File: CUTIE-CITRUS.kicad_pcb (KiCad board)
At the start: 2 copper layers, 31 parts, among them J1 F32Q-1A7H1-11022, J2 F32Q-1A7H1-11022, J3 Bus_M.2_Socket_M, U1 ASEK-32.768KHZ-L-R-T, U2 AP3441SHE-7B, U3 ICM-42688-P, U4 NEO-M8M

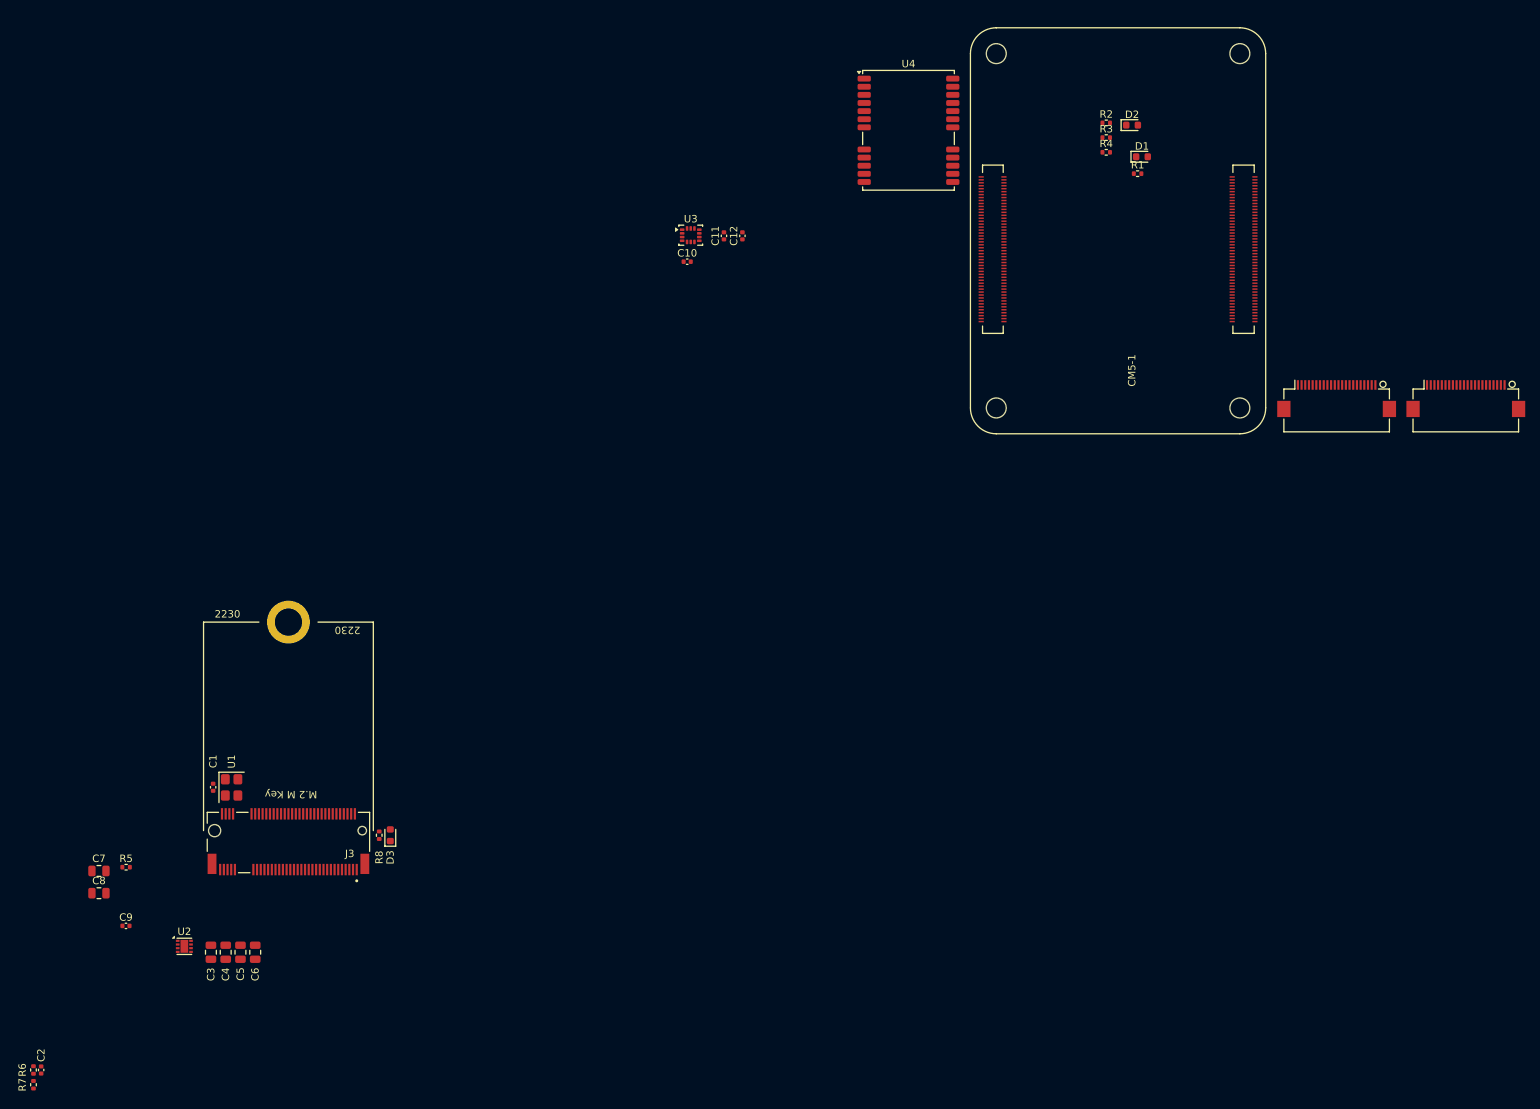
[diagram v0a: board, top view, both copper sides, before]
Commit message: neo m8m impl.
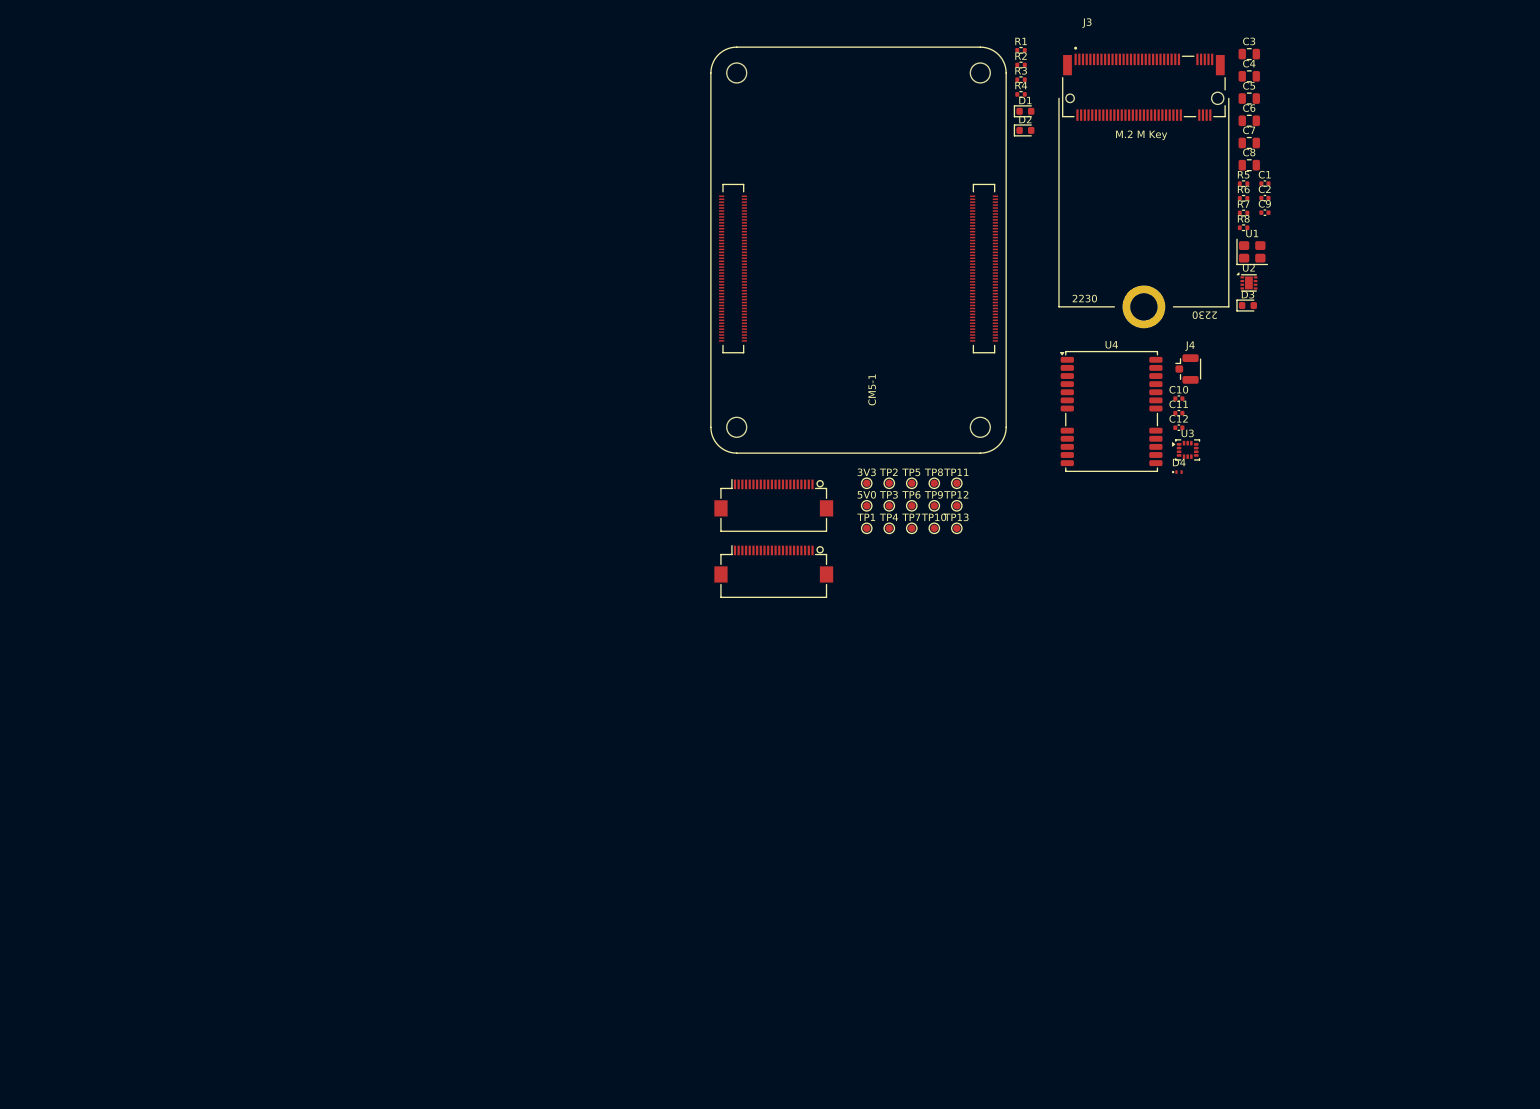
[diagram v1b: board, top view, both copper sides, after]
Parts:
- added 3V3: TestPoint, TestPoint:TestPoint_Pad_D1.0mm, F.Cu at (136.3, 110.5)
- added 5V0: TestPoint, TestPoint:TestPoint_Pad_D1.0mm, F.Cu at (136.3, 113.6)
- added D4: TPD1E05U06DPY, Package_SON:Texas_DPY0002A_0.6x1mm_P0.65mm, F.Cu at (178.7, 109.0)
- added J4: Hirose U.FL, Connector_Coaxial:U.FL_Hirose_U.FL-R-SMT-1_Vertical, F.Cu at (179.7, 95.0)
- added TP1: TestPoint, TestPoint:TestPoint_Pad_D1.0mm, F.Cu at (136.3, 116.6)
- added TP10: TestPoint, TestPoint:TestPoint_Pad_D1.0mm, F.Cu at (145.5, 116.6)
- added TP11: TestPoint, TestPoint:TestPoint_Pad_D1.0mm, F.Cu at (148.5, 110.5)
- added TP12: TestPoint, TestPoint:TestPoint_Pad_D1.0mm, F.Cu at (148.5, 113.6)
- added TP13: TestPoint, TestPoint:TestPoint_Pad_D1.0mm, F.Cu at (148.5, 116.6)
- added TP2: TestPoint, TestPoint:TestPoint_Pad_D1.0mm, F.Cu at (139.4, 110.5)
- added TP3: TestPoint, TestPoint:TestPoint_Pad_D1.0mm, F.Cu at (139.4, 113.6)
- added TP4: TestPoint, TestPoint:TestPoint_Pad_D1.0mm, F.Cu at (139.4, 116.6)
- added TP5: TestPoint, TestPoint:TestPoint_Pad_D1.0mm, F.Cu at (142.4, 110.5)
- added TP6: TestPoint, TestPoint:TestPoint_Pad_D1.0mm, F.Cu at (142.4, 113.6)
- added TP7: TestPoint, TestPoint:TestPoint_Pad_D1.0mm, F.Cu at (142.4, 116.6)
- added TP8: TestPoint, TestPoint:TestPoint_Pad_D1.0mm, F.Cu at (145.5, 110.5)
- added TP9: TestPoint, TestPoint:TestPoint_Pad_D1.0mm, F.Cu at (145.5, 113.6)
- moved C2 203.6 mm to (190.3, 71.9), turned to 0 degrees
- moved R7 202.0 mm to (187.4, 73.9), turned to 0 degrees
- moved R6 202.0 mm to (187.4, 71.9), turned to 0 degrees
- moved C3 186.0 mm to (188.2, 52.4), turned to 0 degrees
- moved C7 184.4 mm to (188.2, 64.4)
- moved C8 184.4 mm to (188.2, 67.4)
- moved C4 182.5 mm to (188.2, 55.4), turned to 0 degrees
- moved C9 182.1 mm to (190.3, 73.9)
- moved C5 179.0 mm to (188.2, 58.4), turned to 0 degrees
- moved R5 177.5 mm to (187.4, 69.9)
- moved C6 175.6 mm to (188.2, 61.4), turned to 0 degrees
- moved U2 169.9 mm to (188.1, 83.4)
- moved C1 164.3 mm to (190.3, 69.9), turned to 0 degrees
- moved U1 156.1 mm to (188.6, 79.2), turned to 0 degrees
- moved J3 152.6 mm to (173.9, 58.4), turned to 0 degrees
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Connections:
- net /CM5/5V0 renamed /NVME/5V0
- net /CM5/I2C0.SCL renamed /Cameras/I2C0.SCL
- net /CM5/I2C0.SDA renamed /Cameras/I2C0.SDA
- net /CM5/PCIE_PWR_EN renamed /CM5/PCIEsb.PWR_EN
- net /CM5/PCIE_nCLKREQ renamed /CM5/PCIEsb.nCLKREQ
- net /CM5/PCIE_nRST renamed /CM5/PCIEsb.nRST
- net /CM5/PCIE_nWAKE renamed /CM5/PCIEsb.nWAKE
- net /CM5/VBUS_EN renamed /CM5/High-Speed Serial/VBUS_EN
- C10 pad 1: /CM5/3V3 -> /Cameras/3V3
- C11 pad 1: /CM5/3V3 -> /Cameras/3V3
- C12 pad 1: /CM5/3V3 -> /Cameras/3V3
- CM5-1 pad 100: GND -> /CM5/CAM_GPIO1
- CM5-1 pad 78: /CM5/3V3 -> /Cameras/3V3
- CM5-1 pad 80: GND -> /CM5/GPIO/I2C0.SCL
- CM5-1 pad 82: GND -> /CM5/GPIO/I2C0.SDA
- CM5-1 pad 84: /CM5/3V3 -> /Cameras/3V3
- CM5-1 pad 86: /CM5/3V3 -> /Cameras/3V3
- D1 pad 2: /CM5/3V3 -> /Cameras/3V3
- D2 pad 2: /CM5/3V3 -> /Cameras/3V3
- J1 pad 18: GND -> /CM5/CAM_GPIO1
- J1 pad 22: /CM5/3V3 -> /Cameras/3V3
- J2 pad 22: /CM5/3V3 -> /Cameras/3V3
- R2 pad 1: /CM5/3V3 -> /Cameras/3V3
- R3 pad 1: /CM5/3V3 -> /Cameras/3V3
- U3 pad 5: /CM5/3V3 -> /Cameras/3V3
- U3 pad 8: /CM5/3V3 -> /Cameras/3V3
- U4 pad 10: Net-(U4-GND-Pad10) -> GND
- U4 pad 11: unconnected-(U4-RF_IN-Pad11) -> Net-(U4-RF_IN)
- U4 pad 12: Net-(U4-GND-Pad10) -> Net-(U4-GND-Pad12)
- U4 pad 13: Net-(U4-GND-Pad10) -> Net-(U4-GND-Pad12)
- U4 pad 18: unconnected-(U4-SDA/~{SPI_CS}-Pad18) -> /CM5/SPI0.CS1n
- U4 pad 19: unconnected-(U4-SCL/SPI_CLK-Pad19) -> /CM5/SPI0.SCLK
- U4 pad 20: unconnected-(U4-TXD/SPI_MISO-Pad20) -> /CM5/SPI0.MISO
- U4 pad 21: unconnected-(U4-RXD/SPI_MOSI-Pad21) -> /CM5/SPI0.MOSI
- U4 pad 22: unconnected-(U4-V_BCKP-Pad22) -> /Cameras/3V3
- U4 pad 23: unconnected-(U4-VCC-Pad23) -> /Cameras/3V3
- U4 pad 24: Net-(U4-GND-Pad10) -> Net-(U4-GND-Pad12)
- U4 pad 7: unconnected-(U4-VDD_USB-Pad7) -> GND
